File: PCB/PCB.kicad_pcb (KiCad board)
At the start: 2 copper layers, 70 parts, among them J1 USB_C_Receptacle_USB2.0_14P, J2 OLED_128x64, SW1 SW_Push, SW2 RotaryEncoder, SW3 RotaryEncoder, U1 STM32F072CBTx, U2 USBLC6-2SC6, U3 XC6206, U5 TRRS

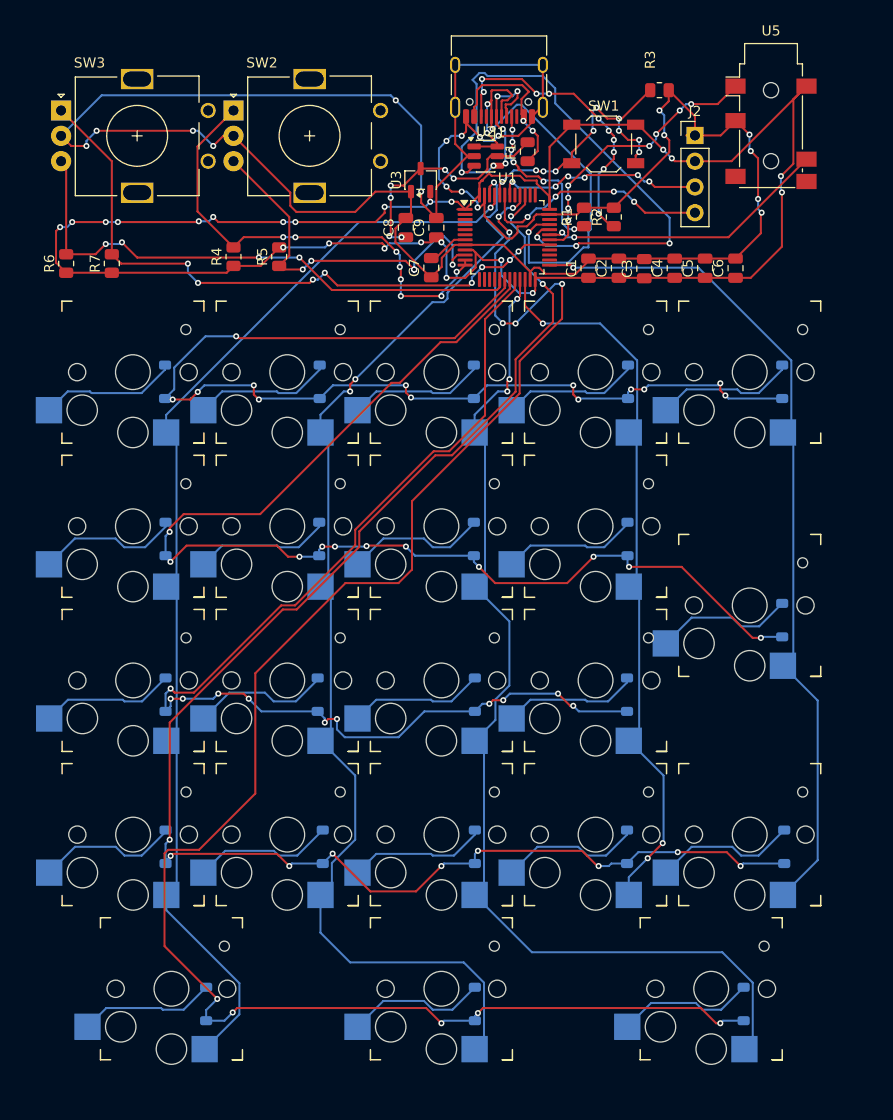
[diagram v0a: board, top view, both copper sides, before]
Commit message: Finally DCR check passed
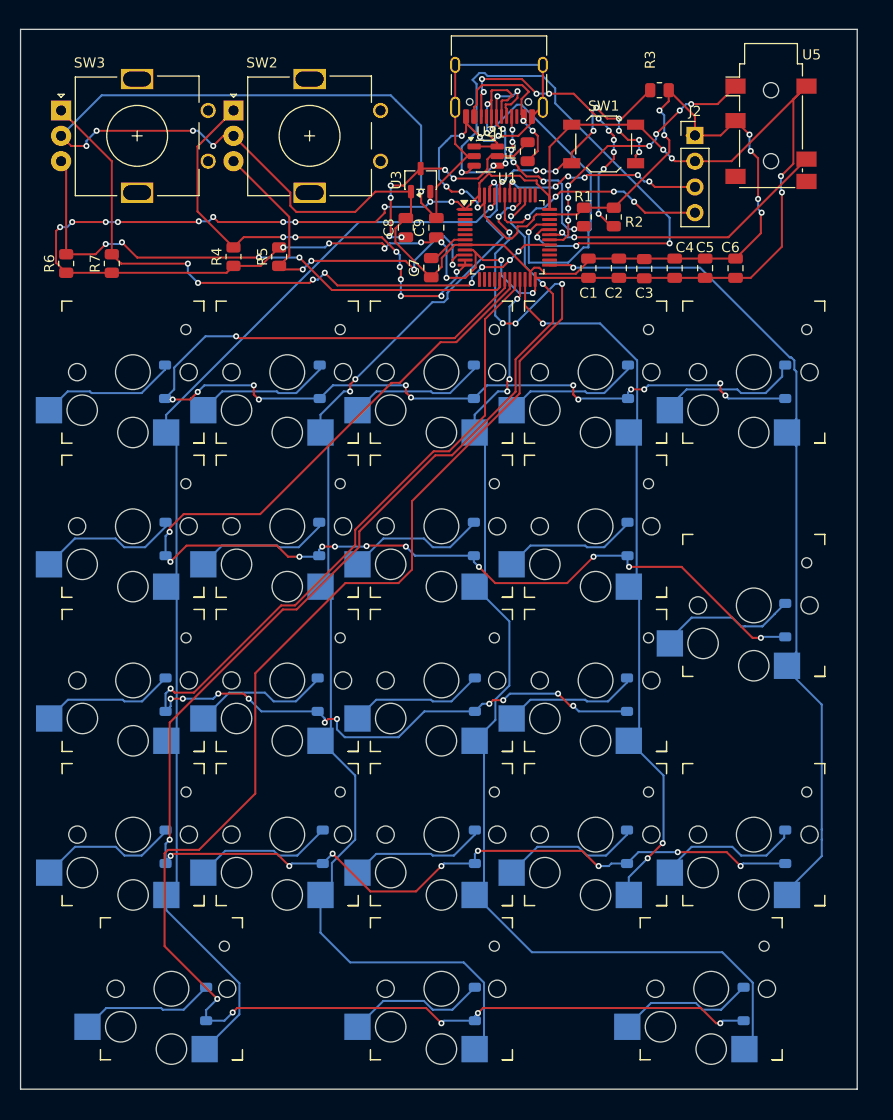
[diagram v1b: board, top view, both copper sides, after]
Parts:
- moved S10 0.40 mm to (109.3, 86.8)
- moved S22 0.40 mm to (109.3, 109.4)
- moved S5 0.40 mm to (109.3, 63.8)
- moved D10 0.30 mm to (112.4, 88.2)
- moved D5 0.30 mm to (112.4, 64.8)
- moved D22 0.10 mm to (112.4, 110.6)
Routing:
- net C4: track 84.5 -> 85.6 mm
- net RE_1_A: vias 5 -> 4
- net GND: vias 19 -> 17
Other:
- board outline added: 82.5 x 104.5 mm

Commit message: Updated the PCB with proper alignments and design decisions
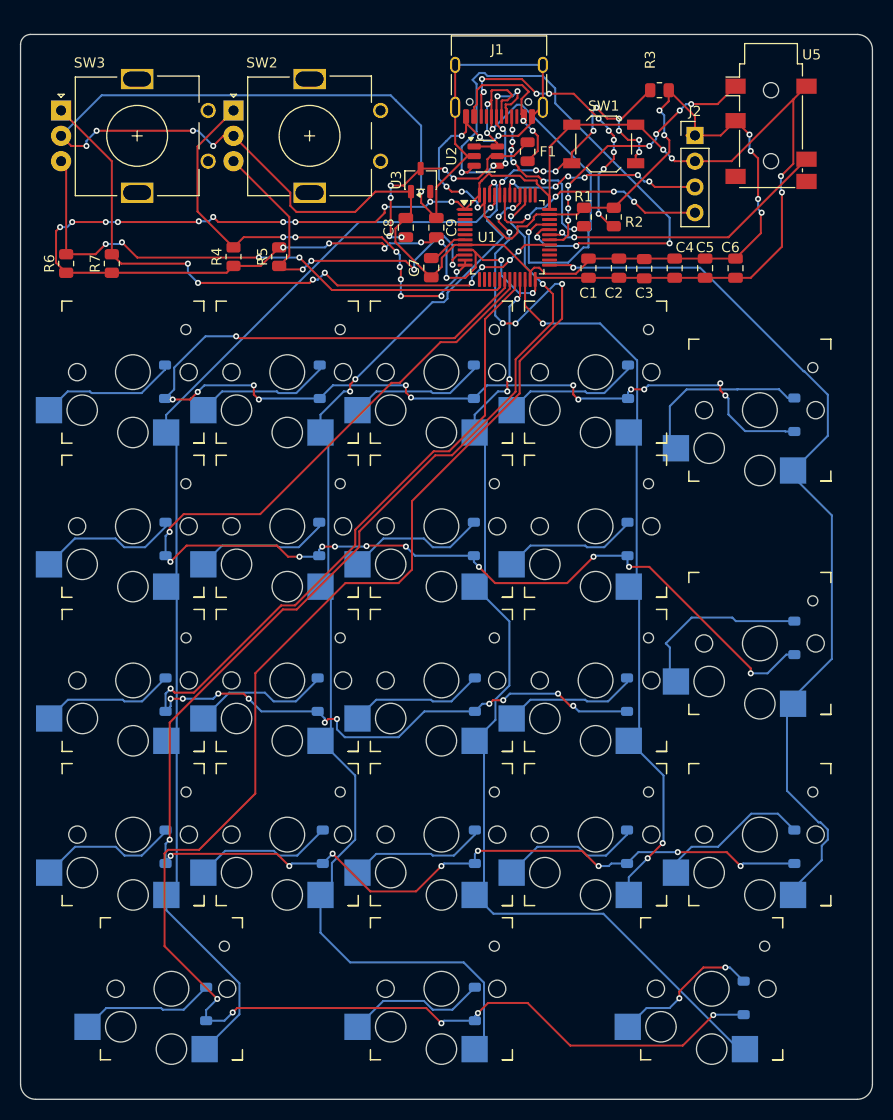
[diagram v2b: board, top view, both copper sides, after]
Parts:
- moved S10 3.80 mm to (109.9, 90.5)
- moved S5 3.80 mm to (109.9, 67.5)
- moved D5 3.37 mm to (113.3, 68.0)
- moved D10 1.97 mm to (113.3, 90.0)
- moved D22 0.90 mm to (113.3, 110.6)
- moved S22 0.60 mm to (109.9, 109.4)
- moved D21 0.60 mm to (108.3, 125.5)
- moved S21 0.05 mm to (105.2, 124.6)
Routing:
- net C4: track 85.6 -> 92.0 mm
- net C2: track 105.4 -> 100.5 mm
- net Net-(D10-A): track 14.0 -> 17.8 mm
- net R1: track 117.1 -> 120.8 mm
- net R0: track 108.1 -> 111.5 mm
- net Net-(D5-A): track 14.3 -> 17.5 mm
- net R4: track 174.8 -> 177.3 mm
- net +3.3V: track 199.5 -> 197.7 mm
- net Net-(D22-A): track 14.6 -> 15.8 mm
- net Net-(D21-A): track 13.6 -> 14.8 mm, vias 0 -> 2
- net R3: track 154.1 -> 155.1 mm
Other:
- board size 82.5 x 104.5 mm -> 84 x 105 mm
